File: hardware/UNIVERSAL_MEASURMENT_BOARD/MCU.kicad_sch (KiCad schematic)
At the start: 8 parts, among them U1 ADS8863IDGS, U6 STM32G484RET3, Y1 ECS-1612MV

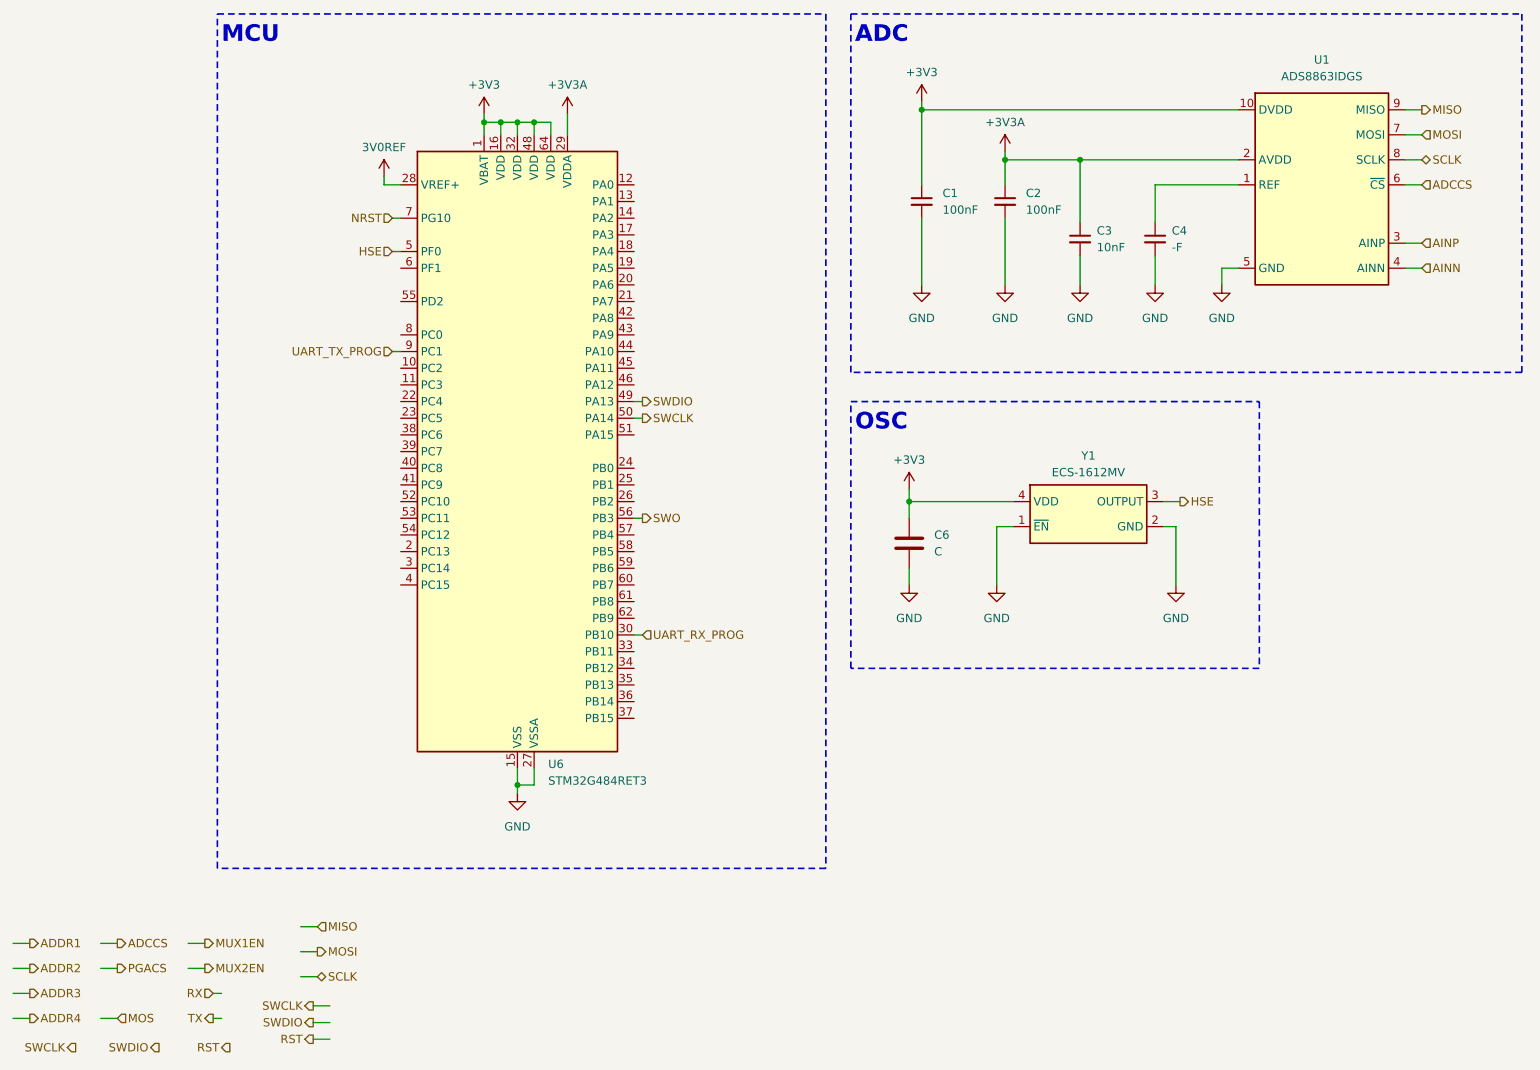
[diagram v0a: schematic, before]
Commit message: final schematic review corrections
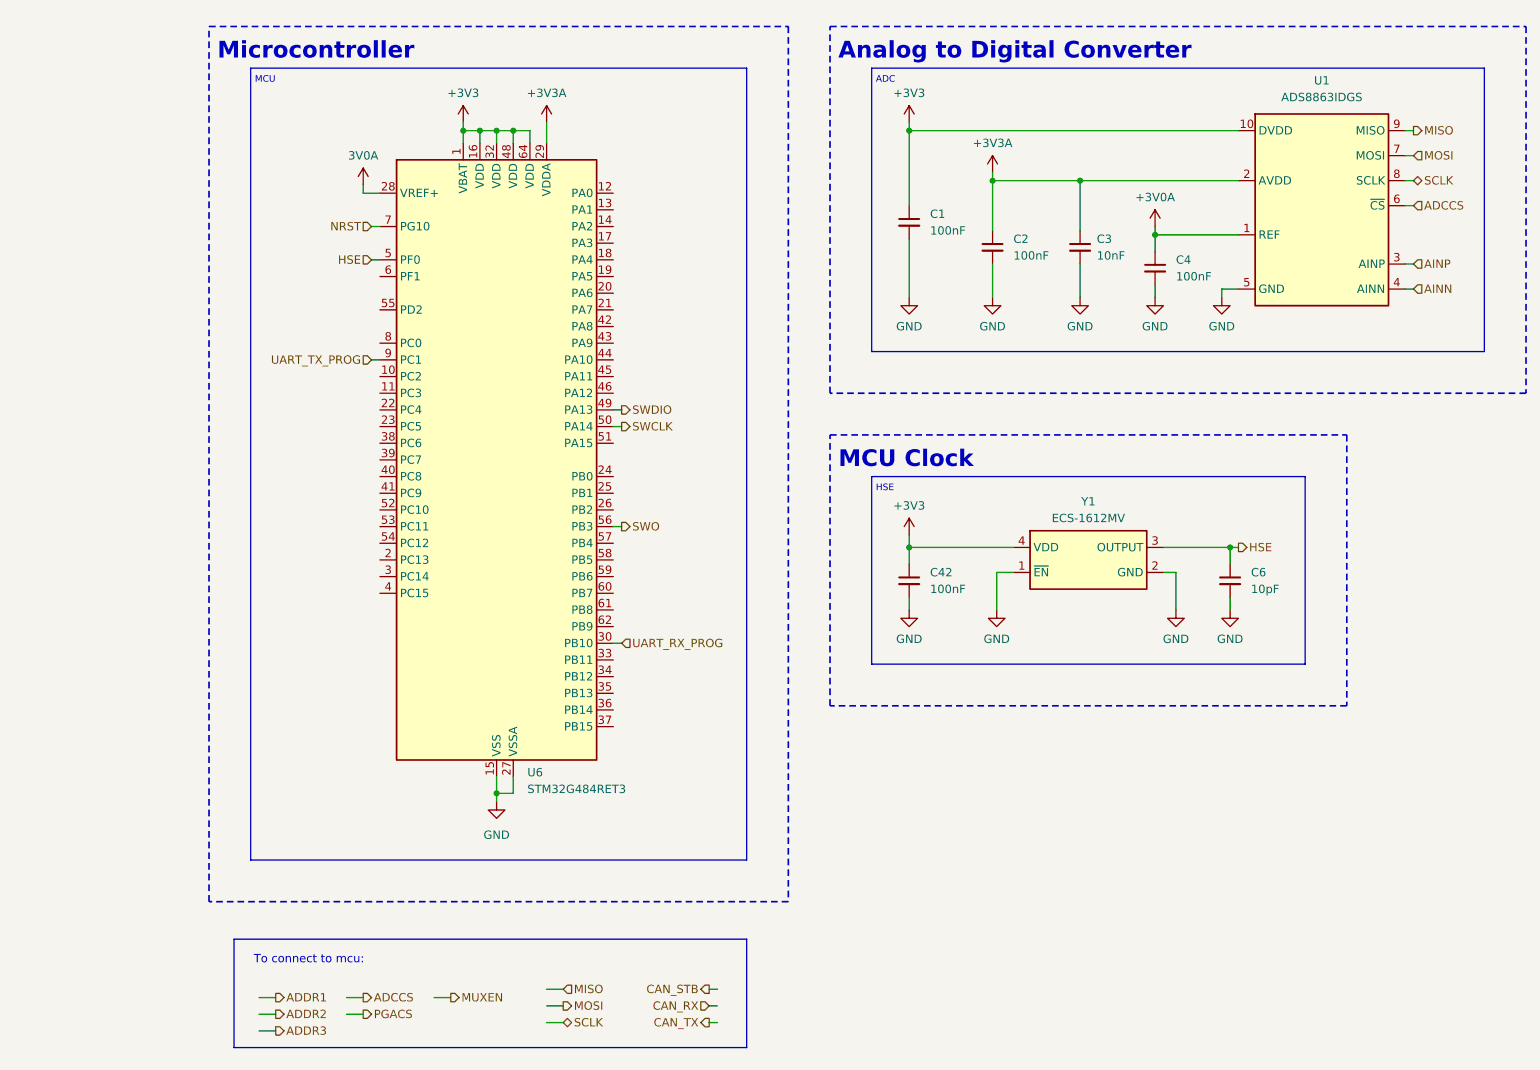
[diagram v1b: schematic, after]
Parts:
- removed C6: C, symbol Device:C
- added C42: 100nF, symbol Device:C_Small
- added C6: 10pF, symbol Device:C_Small
- C4: value -F -> 100nF
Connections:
- net +3V3: now also C42.1
- net GND: now also C42.2, C6.2
- net HSE: now also C6.1
- net +3V0A: now reaches C4.1, U1.1 (REF)
- net 3V0REF renamed 3V0A
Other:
- note added: "Analog to Digital Converter"
- note added: "HSE"
- note added: "MCU Clock"
- note added: "Microcontroller"
- note added: "To connect to mcu:"
- note removed: "OSC"
- moved on the sheet: C1, C2, C3, C4, U1, U6, Y1
